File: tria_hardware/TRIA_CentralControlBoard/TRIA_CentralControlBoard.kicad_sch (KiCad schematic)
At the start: 6 parts, among them J5 resistor_enable, U9 MCP2562-E-P

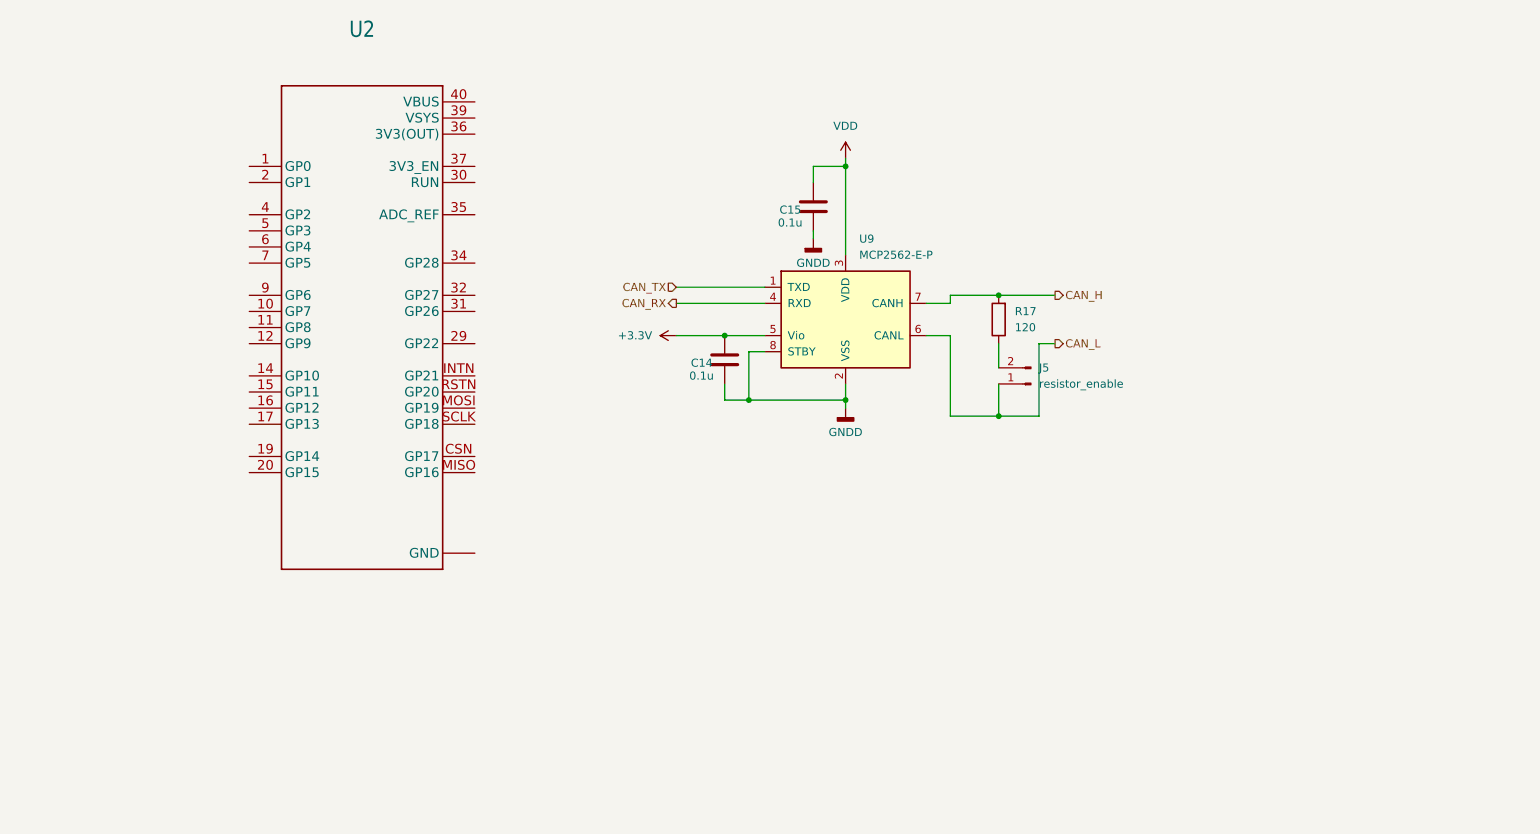
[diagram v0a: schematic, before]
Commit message: [update] 基板データのアップデート
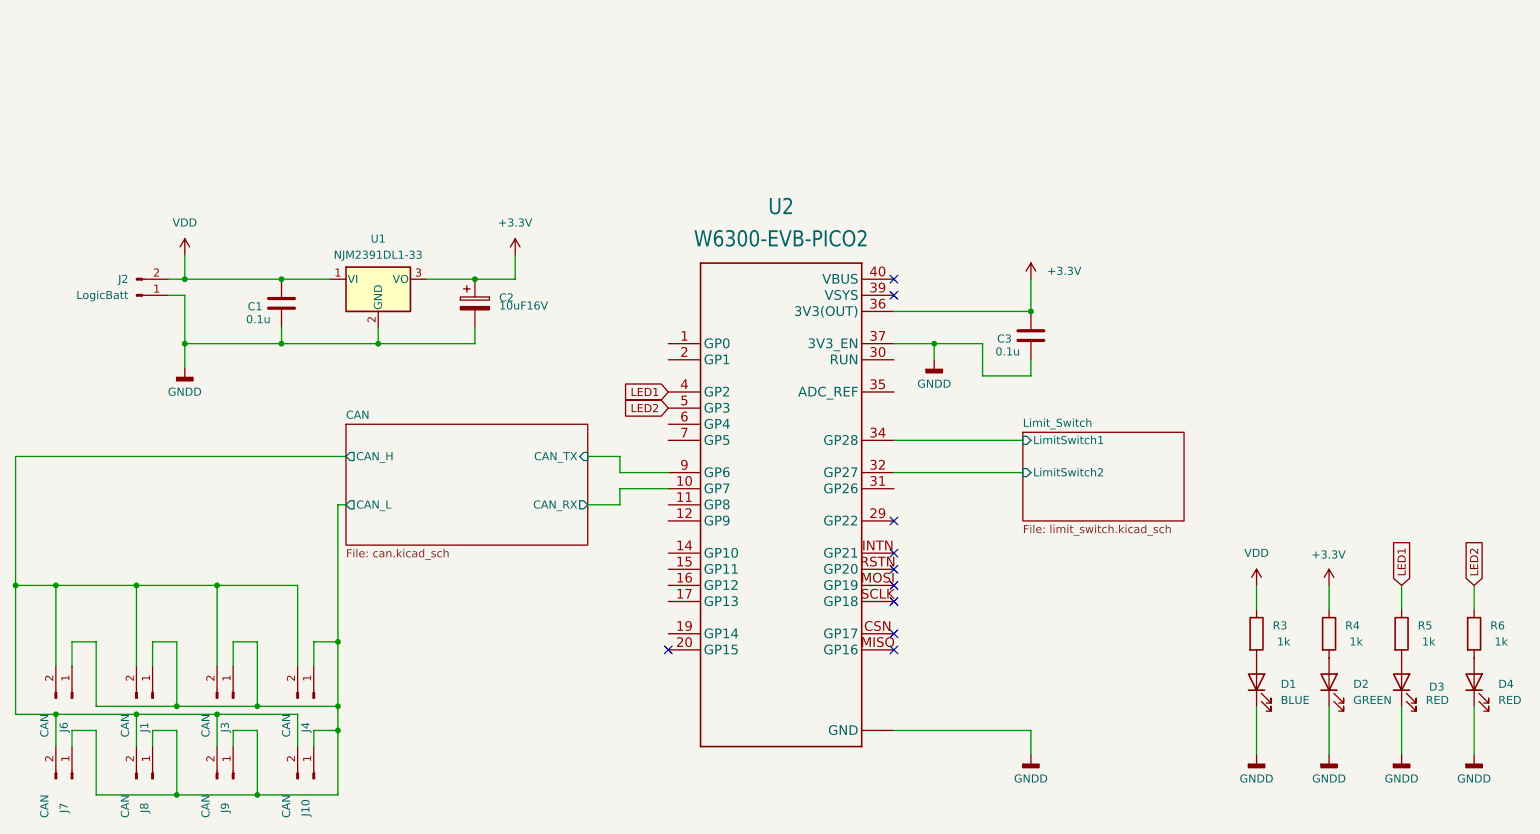
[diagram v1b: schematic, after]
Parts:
- removed C14, C15: 0.1u, Capacitor_THT:C_Disc_D3.0mm_W1.6mm_P2.50mm, symbol Device:C
- removed J5: resistor_enable, Connector_PinHeader_2.54mm:PinHeader_1x02_P2.54mm_Vertical, symbol Connector:Conn_01x02_Pin
- removed R17: 120, Resistor_THT:R_Axial_DIN0207_L6.3mm_D2.5mm_P10.16mm_Horizontal, symbol Device:R
- removed U9: MCP2562-E-P, Package_DIP:DIP-8_W7.62mm, symbol Interface_CAN_LIN:MCP2562-E-P
- added C1, C3: 0.1u, Capacitor_THT:C_Disc_D3.0mm_W1.6mm_P2.50mm, symbol Device:C
- added C2: 10uF16V, Capacitor_THT:CP_Radial_D4.0mm_P1.50mm, symbol Device:C_Polarized
- added D1: BLUE, LED_THT:LED_D3.0mm, symbol Device:LED
- added D2: GREEN, LED_THT:LED_D3.0mm, symbol Device:LED
- added D3, D4: RED, LED_THT:LED_D3.0mm, symbol Device:LED
- added J1, J10, J3, J4, J6, J7, J8, J9: CAN, Connector_JST:JST_XH_B2B-XH-A_1x02_P2.50mm_Vertical, symbol Connector:Conn_01x02_Pin
- added J2: LogicBatt, Connector_AMASS:AMASS_XT30U-M_1x02_P5.0mm_Vertical, symbol Connector:Conn_01x02_Pin
- added R3, R4, R5, R6: 1k, Resistor_THT:R_Axial_DIN0207_L6.3mm_D2.5mm_P10.16mm_Horizontal, symbol Device:R
- added U1: NJM2391DL1-33, Package_TO_SOT_SMD:TO-252-2, symbol Regulator_Linear:LM7805_TO220
- U2: value ~ -> W6300-EVB-PICO2
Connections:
- net +3.3V: now also U2.36 (3V3(OUT)), C2.1, C3.1, R4.1, U1.3 (VO)
- net GNDD: now also U2.13 (GND), U2.18 (GND), U2.23 (GND), U2.28 (GND), U2.3 (GND), U2.33 (GND), U2.37 (3V3_EN), U2.38 (GND), U2.8 (GND), C1.2, C2.2, C3.2, D1.1 (K), D2.1 (K), D3.1 (K), D4.1 (K), J2.1 (Pin_1), U1.2 (GND)
- net VDD: now also C1.1, J2.2 (Pin_2), R3.1, U1.1 (VI)
- net CAN/CAN_RX: now reaches U2.10 (GP7)
- net Limit_Switch/LimitSwitch2: now reaches U2.32 (GP27)
- net Limit_Switch/LimitSwitch1: now reaches U2.34 (GP28)
- net LED1: now reaches U2.4 (GP2)
- net LED1: now also R5.1
- net LED2: now reaches U2.5 (GP3)
- net LED2: now also R6.1
- net CAN/CAN_TX: now reaches U2.9 (GP6)
- new net: D4.2 (A), R6.2
- new net: D1.2 (A), R3.2
- new net: D3.2 (A), R5.2
- new net: D2.2 (A), R4.2
- new net CAN/CAN_H: J1.2 (Pin_2), J10.2 (Pin_2), J3.2 (Pin_2), J4.2 (Pin_2), J6.2 (Pin_2), J7.2 (Pin_2), J8.2 (Pin_2), J9.2 (Pin_2)
- new net CAN/CAN_L: J1.1 (Pin_1), J10.1 (Pin_1), J3.1 (Pin_1), J4.1 (Pin_1), J6.1 (Pin_1), J7.1 (Pin_1), J8.1 (Pin_1), J9.1 (Pin_1)
- no-connect marks 0 -> 10
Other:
- added sheet CAN (can.kicad_sch)
- added sheet Limit_Switch (limit_switch.kicad_sch)
- moved on the sheet: U2
